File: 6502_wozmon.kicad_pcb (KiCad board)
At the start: 2 copper layers, 186.8 x 132.7 mm, 38 parts, among them J1 Barrel_Jack_Switch_Pin3Ring, J2 DB9_Female, J3 "Switch", J4 Conn_01x08_Male, U1 7400, U2 W65C02, U3 28C256, U4 W65C51N, U5 62256, U6 MAX232, U7 65C22, U8 WC1602A, X1 GTXO-S14V, Y1 1.8432MHZ

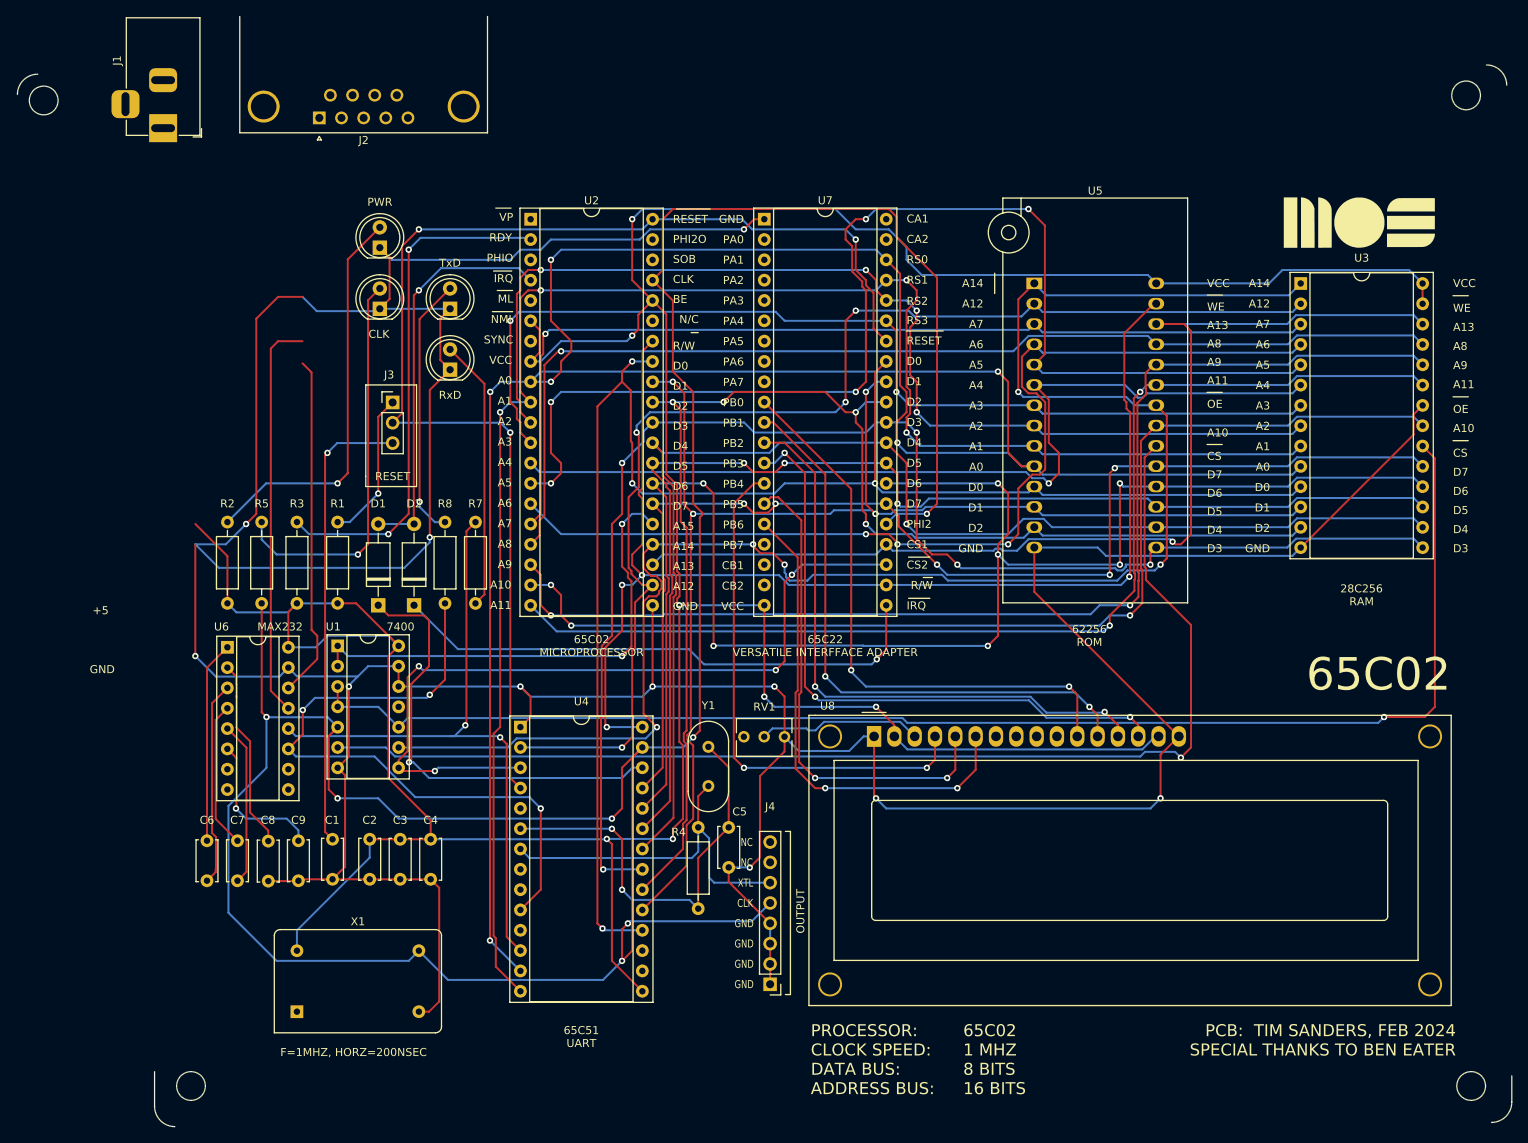
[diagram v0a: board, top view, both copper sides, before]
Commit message: increment
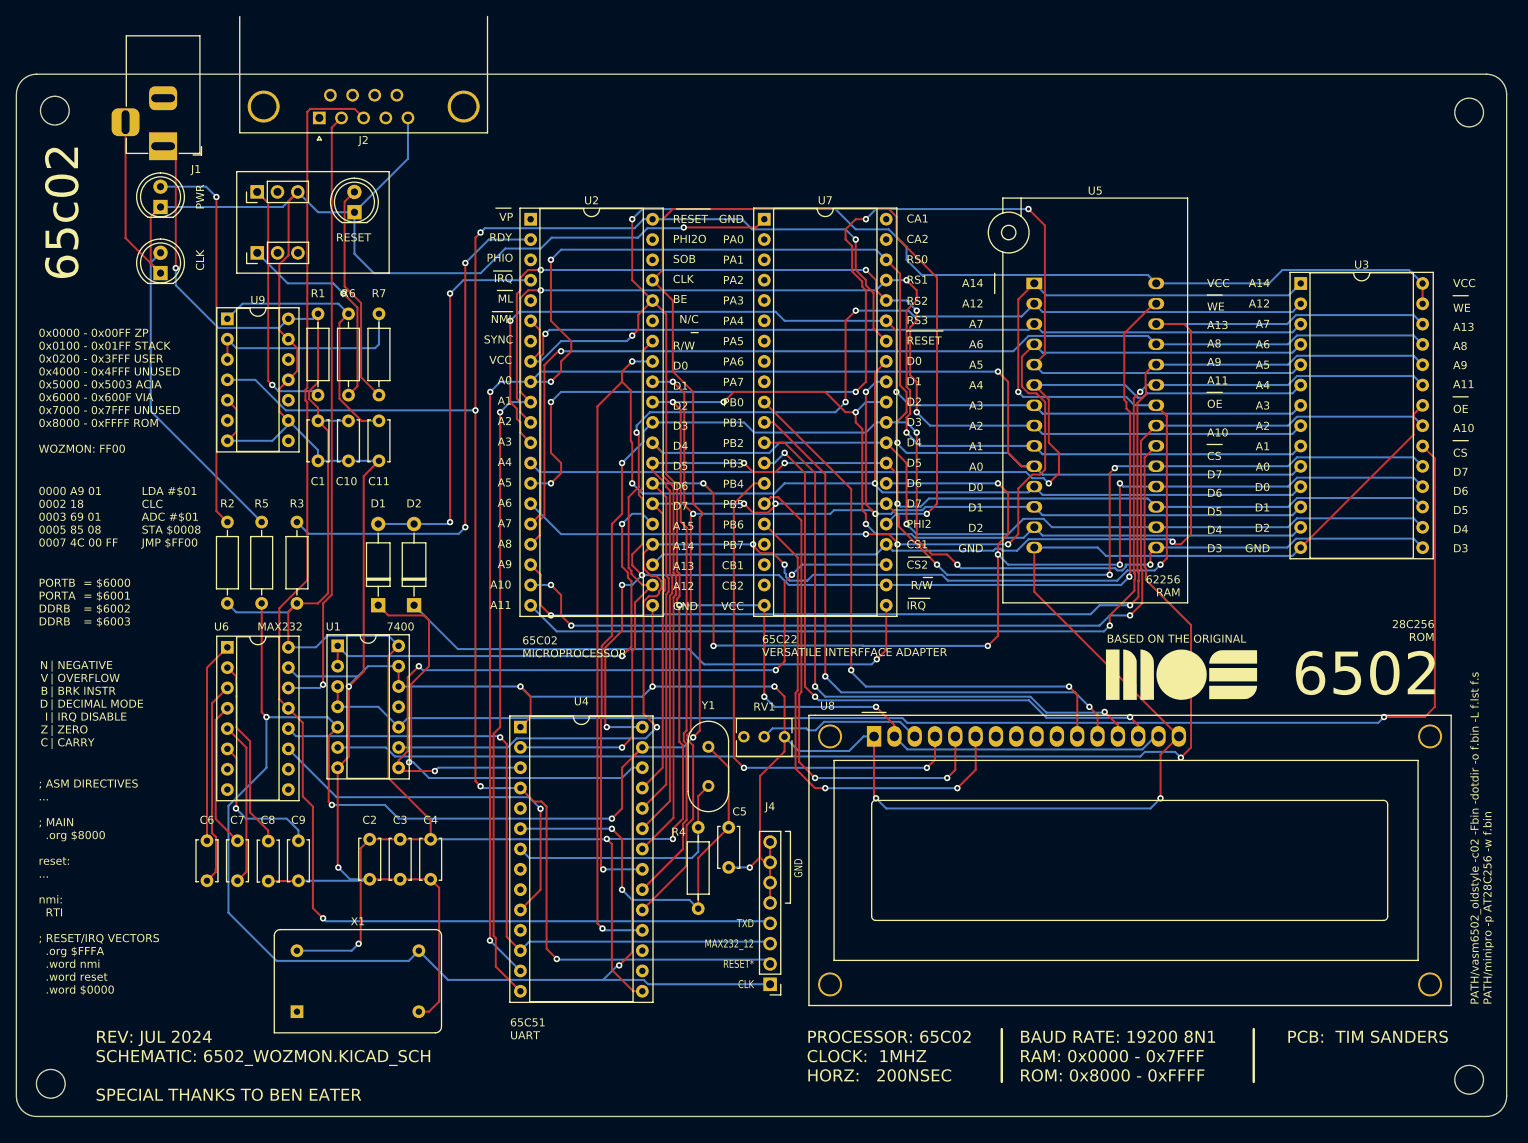
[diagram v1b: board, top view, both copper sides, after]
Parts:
- removed LED_3, LED_4: LED, LED_THT:LED_D5.0mm
- removed R8: 220, Resistor_THT:R_Axial_DIN0207_L6.3mm_D2.5mm_P10.16mm_Horizontal
- added C10: C, Capacitor_THT:C_Disc_D5.0mm_W2.5mm_P5.00mm, F.Cu at (56.5, 59.1)
- added C11: 10u, Capacitor_THT:C_Disc_D5.0mm_W2.5mm_P5.00mm, F.Cu at (60.3, 59.1)
- added D3: LED, LED_THT:LED_D5.0mm, F.Cu at (57.3, 33.0)
- added J5: Conn_01x03_Male, Connector_PinHeader_2.54mm:PinHeader_1x03_P2.54mm_Vertical, F.Cu at (45.1, 30.5)
- added R6: 1K, Resistor_THT:R_Axial_DIN0207_L6.3mm_D2.5mm_P10.16mm_Horizontal, F.Cu at (56.5, 55.9)
- added U9: 74HC14, Package_DIP:DIP-14_W7.62mm_Socket, F.Cu at (41.4, 46.4)
- C1: value 0.1u -> C
- J3: value "Switch" -> Conn_01x03_Male
- R1: value 1K -> 10K
- R7: value 220 -> 330
- moved G*** 60.7 mm to (160.7, 90.8)
- moved C1 57.3 mm to (52.7, 59.1), turned to -90 degrees
- moved R7 28.7 mm to (60.3, 45.7)
- moved LED_1 27.9 mm to (33.0, 32.4)
- moved LED_2 27.8 mm to (33.0, 40.6)
- moved R1 26.1 mm to (52.7, 55.9)
- moved J3 25.2 mm to (45.1, 38.1), turned to 90 degrees
- moved J1 2.25 mm to (33.3, 24.8)
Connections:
- C1 pad 1: GND -> VCC
- C1 pad 2: Net-(C1-Pad2) -> GND
- J3 pad 2: RESET* -> unconnected-(J3-Pad2)
- J3 pad 3: Net-(C1-Pad2) -> unconnected-(J3-Pad3)
- J4 pad 1: GND -> CLK
- J4 pad 2: GND -> RESET*
- J4 pad 3: GND -> MAX232_12
- J4 pad 4: GND -> TXD
- J4 pad 5: CLK -> GND
- J4 pad 6: XTAL -> GND
- J4 pad 7: unconnected-(J4-Pad7) -> GND
- J4 pad 8: unconnected-(J4-Pad8) -> GND
- R1 pad 1: VCC -> Net-(J5-Pad1)
- R1 pad 2: Net-(J3-Pad1) -> VCC
- U4 pad 12: Net-(R7-Pad1) -> MAX232_12
- U6 pad 12: Net-(R7-Pad1) -> MAX232_12
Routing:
- net TXD: track 50.2 -> 168.5 mm, vias 0 -> 1
- net MAX232_12: track 0.00 -> 86.4 mm, vias 0 -> 1
- net RESET*: track 156.2 -> 221.1 mm, vias 3 -> 5
- net VCC: track 450.3 -> 511.9 mm, vias 7 -> 9
- net Net-(C1-Pad2): track 57.5 -> 0.00 mm, vias 1 -> 0
- net Net-(R7-Pad1): track 82.9 -> 26.0 mm, vias 2 -> 0
- net Net-(U4-Pad10): track 82.9 -> 48.3 mm, vias 3 -> 1
- net Net-(C11-Pad1): track 0.00 -> 33.6 mm
- net RXD: track 42.8 -> 76.3 mm, vias 0 -> 1
- net Net-(LED_4-Pad2): track 32.8 -> 0.00 mm, vias 1 -> 0
- net Net-(J5-Pad1): track 0.00 -> 31.2 mm, vias 0 -> 1
- net XTAL: track 46.5 -> 31.7 mm
- net Net-(LED_2-Pad2): track 49.4 -> 39.9 mm, vias 1 -> 0
- net Net-(J3-Pad1): track 18.7 -> 26.8 mm
- net GND: track 557.1 -> 563.9 mm, vias 11 -> 9
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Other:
- board size 186.8 x 132.7 mm -> 186.3 x 130.3 mm
- board text added: "0000 A9 01 0002 18 0003 69 01 0005 85 08 0007 4C 00 FF"
- board text added: "0x0000 - 0x00FF ZP 0x0100 - 0x01FF STACK 0x0200 - 0x3FFF USER 0x4000 - 0x4FFF UNUSED 0x5000 - 0x5003 ACIA 0x6000 - 0x600F VIA 0x7000 - 0x7FFF UNUSED 0x8000 - 0xFFFF ROM WOZMON: FF00"
- board text added: "28C256 ROM"
- board text added: "62256 RAM"
- board text added: "6502"
- board text added: "65c02"
- board text added: "; ASM DIRECTIVES ... ; MAIN .org $8000 reset: ... nmi: RTI ; RESET/IRQ VECTORS .org $FFFA .word nmi .word reset .word $0000"
- board text added: "= $6000 = $6001 = $6002 = $6003"
- board text added: "BASED ON THE ORIGINAL"
- board text added: "BAUD RATE: 19200 8N1 RAM: 0x0000 - 0x7FFF ROM: 0x8000 - 0xFFFF"
- board text added: "LDA #$01 CLC ADC #$01 STA $0008 JMP $FF00"
- board text added: "MAX232_12"
- board text added: "N V B D I Z C"
- board text added: "PATH/vasm6502_oldstyle -c02 -Fbin -dotdir -o f.bin -L f.lst f.s PATH/minipro -p AT28C256 -w f.bin"
- board text added: "PCB: TIM SANDERS"
- board text added: "PORTB PORTA DDRB DDRB"
- board text added: "PROCESSOR: 65C02 CLOCK: 1MHZ HORZ: 200NSEC"
- board text added: "RESET*"
- board text added: "REV: JUL 2024 SCHEMATIC: 6502_WOZMON.KICAD_SCH SPECIAL THANKS TO BEN EATER"
- board text added: "TXD"
- board text added: "| NEGATIVE | OVERFLOW | BRK INSTR | DECIMAL MODE | IRQ DISABLE | ZERO | CARRY"
- board text removed: "+5"
- board text removed: "28C256 RAM"
- board text removed: "62256 ROM"
- board text removed: "65C02"
- board text removed: "65C02 1 MHZ 8 BITS 16 BITS"
- board text removed: "F=1MHZ, HORZ=200NSEC"
- board text removed: "NC"
- board text removed: "OUTPUT"
- board text removed: "PCB: TIM SANDERS, FEB 2024 SPECIAL THANKS TO BEN EATER"
- board text removed: "PROCESSOR: CLOCK SPEED: DATA BUS: ADDRESS BUS:"
- board text removed: "RxD"
- board text removed: "TxD"
- board text removed: "XTL"
